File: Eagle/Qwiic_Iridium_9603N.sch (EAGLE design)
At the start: 58 parts, among them J1 SS4-10-3.50-X-D, J3 PTH, J6 ISP, J7 U.FL, Q1 DMG3415U-7, Q2 2N2222, U1 ATTINY84-ARDUINO, U2 LTC3225EDDB#TRMPBF

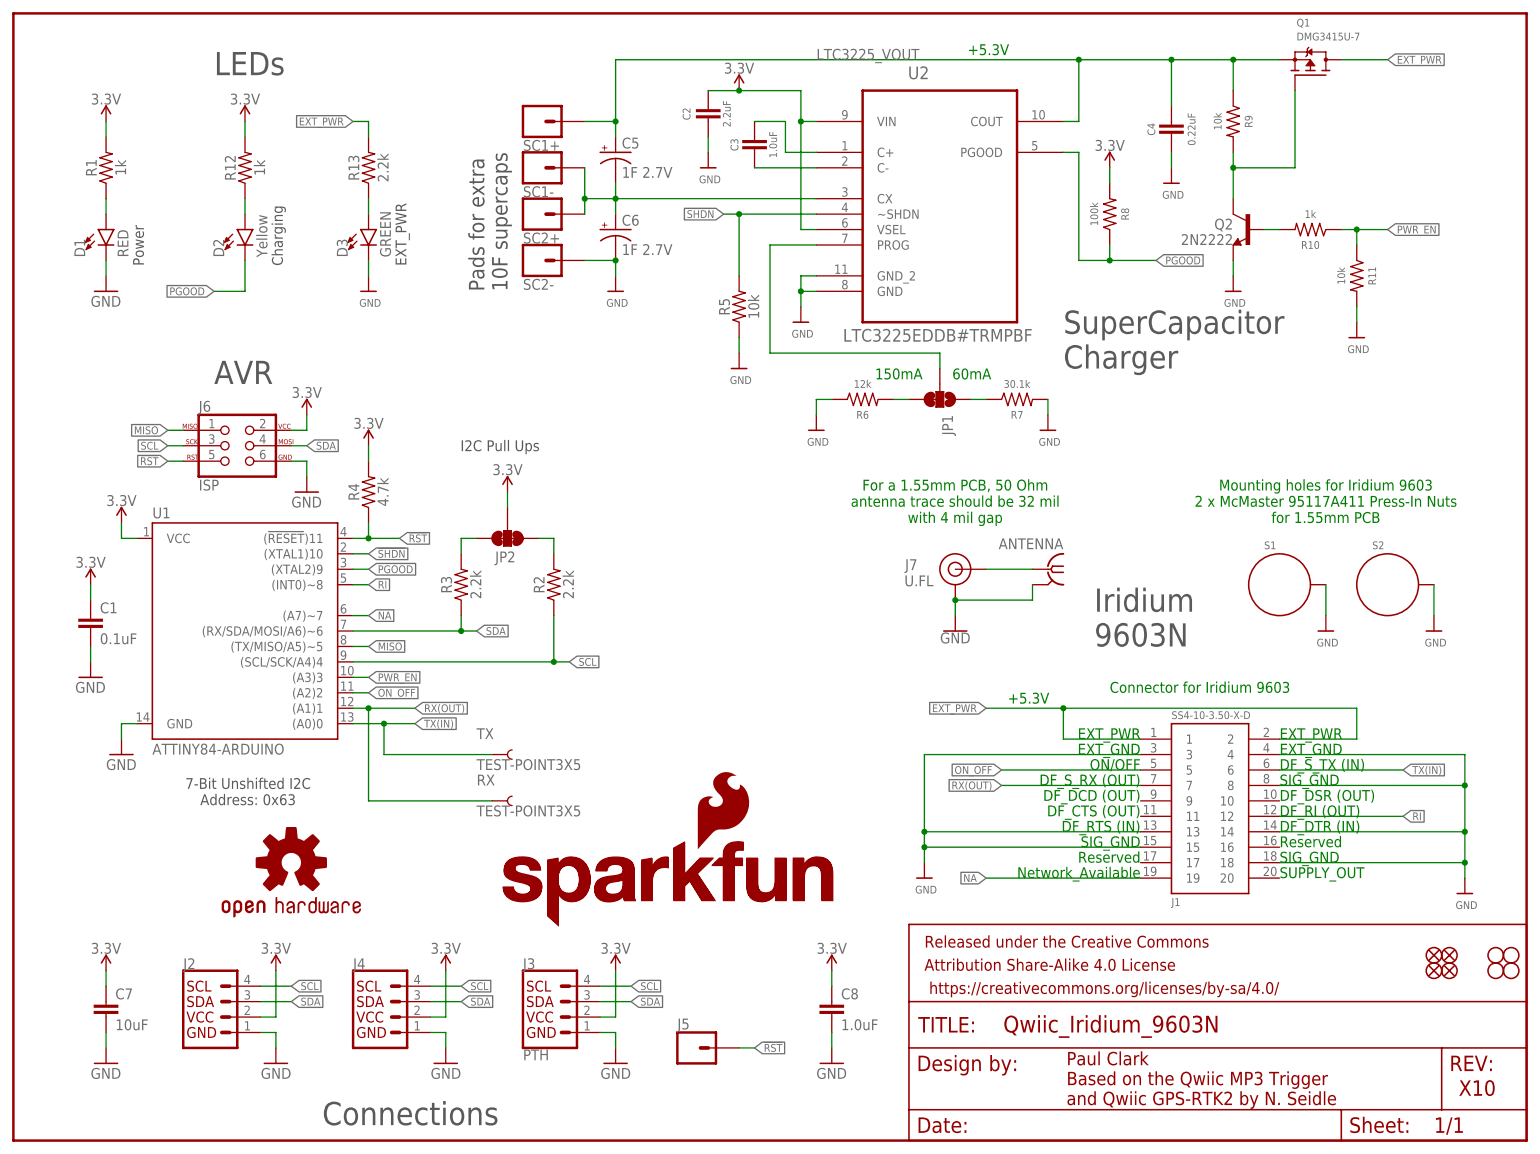
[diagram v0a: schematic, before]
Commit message: Updates for V2 of the PCB
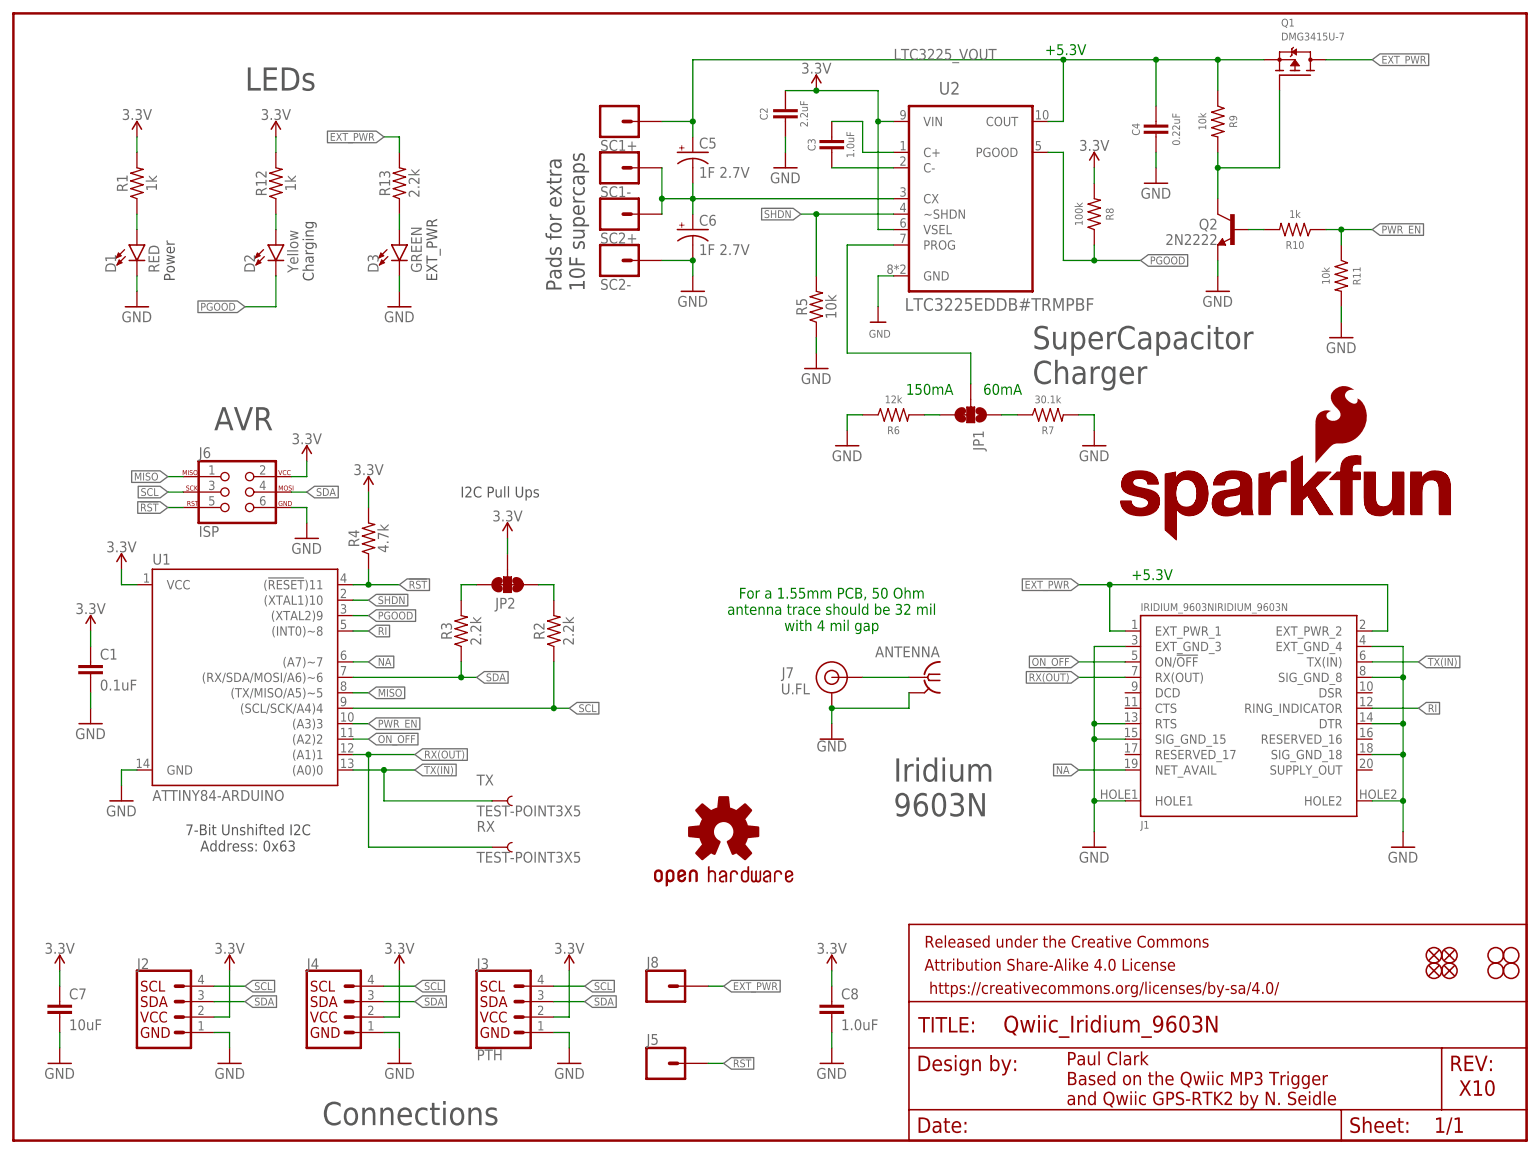
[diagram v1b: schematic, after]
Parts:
- removed S1, S2: STANDOFF_ELECTRICALMCMASTER-95117A411, SparkFun-Electromechanical:STANDOFF_ELECTRICALMCMASTER-95117A411
- added J8: (no value), SparkFun-Connectors:CONN_01PTH_NO_SILK_YES_STOP
- ANTENNA: device con-coax:SMA-142-0711-821/826 -> Qwiic_Iridium_9603N:SMA-142-0711-821/826
- J1: value SS4-10-3.50-X-D -> IRIDIUM_9603NIRIDIUM_9603N; device SS4-10-3.50-X-D:SS4-10-3.50-X-D -> Qwiic_Iridium_9603N:IRIDIUM_9603NIRIDIUM_9603N
- U2: device LTC_By_element14_Batch_1:LTC3225EDDB-TRMPBFDFN300X200-10L -> Qwiic_Iridium_9603N:LTC3225EDDB-TRMPBFDFN300X200-10L
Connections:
- net EXT_PWR: now also J1.EXT_PWR_1, J1.EXT_PWR_2, J8.1; no longer J1.1, J1.2
- net GND: now also J1.DTR, J1.EXT_GND_3, J1.EXT_GND_4, J1.HOLE1, J1.HOLE2, J1.RTS, J1.SIG_GND_15, J1.SIG_GND_18, J1.SIG_GND_8; no longer J1.13, J1.14, J1.15, J1.18, J1.3, J1.4, J1.8, S1.P$1, S2.P$1, U2.GND_2
- net NA: now also J1.NET_AVAIL; no longer J1.19
- net ON_OFF: now also J1.ON/!OFF!; no longer J1.5
- net RI: now also J1.RING_INDICATOR; no longer J1.12
- net RX(OUT): now also J1.RX(OUT); no longer J1.7
- net TX(IN): now also J1.TX(IN); no longer J1.6
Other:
- note removed: "Connector for Iridium 9603"
- note removed: "DF_CTS (OUT)"
- note removed: "DF_DCD (OUT)"
- note removed: "DF_DSR (OUT)"
- note removed: "DF_DTR (IN)"
- note removed: "DF_RI (OUT)"
- note removed: "DF_RTS (IN)"
- note removed: "DF_S_RX (OUT)"
- note removed: "DF_S_TX (IN)"
- note removed: "EXT_GND"
- note removed: "Mounting holes for Iridium 9603 2 x McMaster 95117A411 Press-In Nuts for 1.55mm PCB"
- note removed: "Network_Available"
- note removed: "ON/OFF"
- note removed: "Reserved"
- note removed: "SIG_GND"
- note removed: "SUPPLY_OUT"
- moved on the sheet: ANTENNA, C1, C2, C3, C4, C5, C6, C7, D1, D2, D3, J2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
